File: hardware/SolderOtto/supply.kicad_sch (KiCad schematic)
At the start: 78 parts, among them J201 Conn_02x04_Counter_Clockwise, Q201 T2N7002AK, Q202 BC858B, Q203 BC847A, Q204 BC847A, U201 LM5012, U202 AP3211K, U203 AP3211K, U204 AP3211K, U205 LM27761, U206 MCP9701T-E/TT

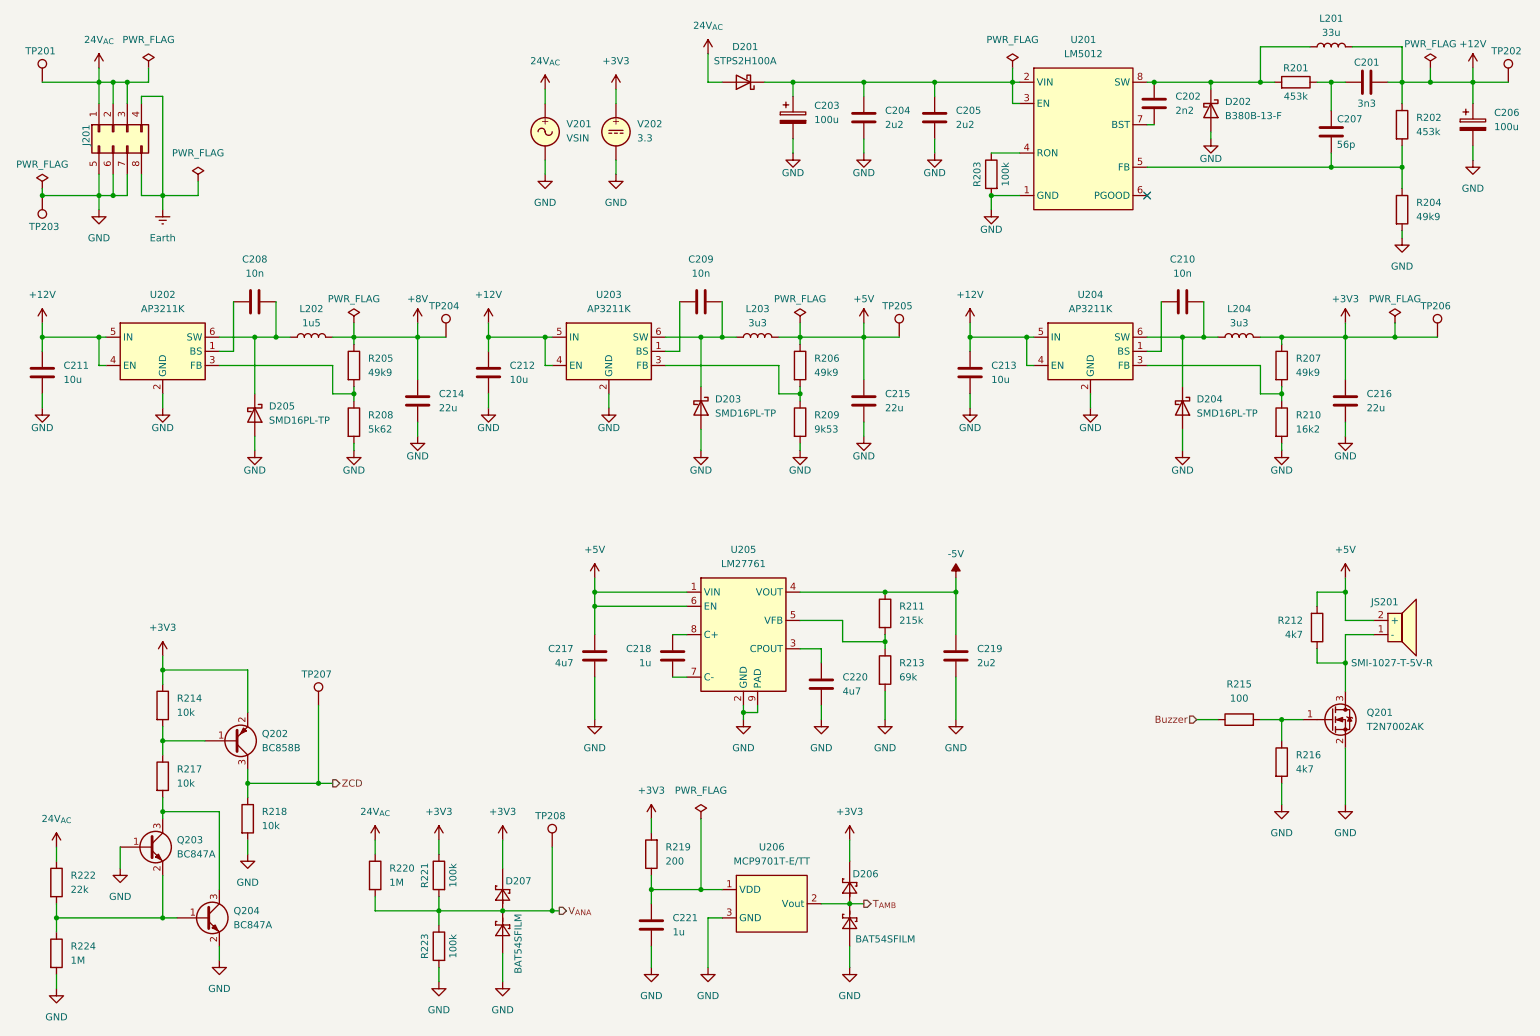
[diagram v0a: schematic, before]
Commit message: start rework supplies
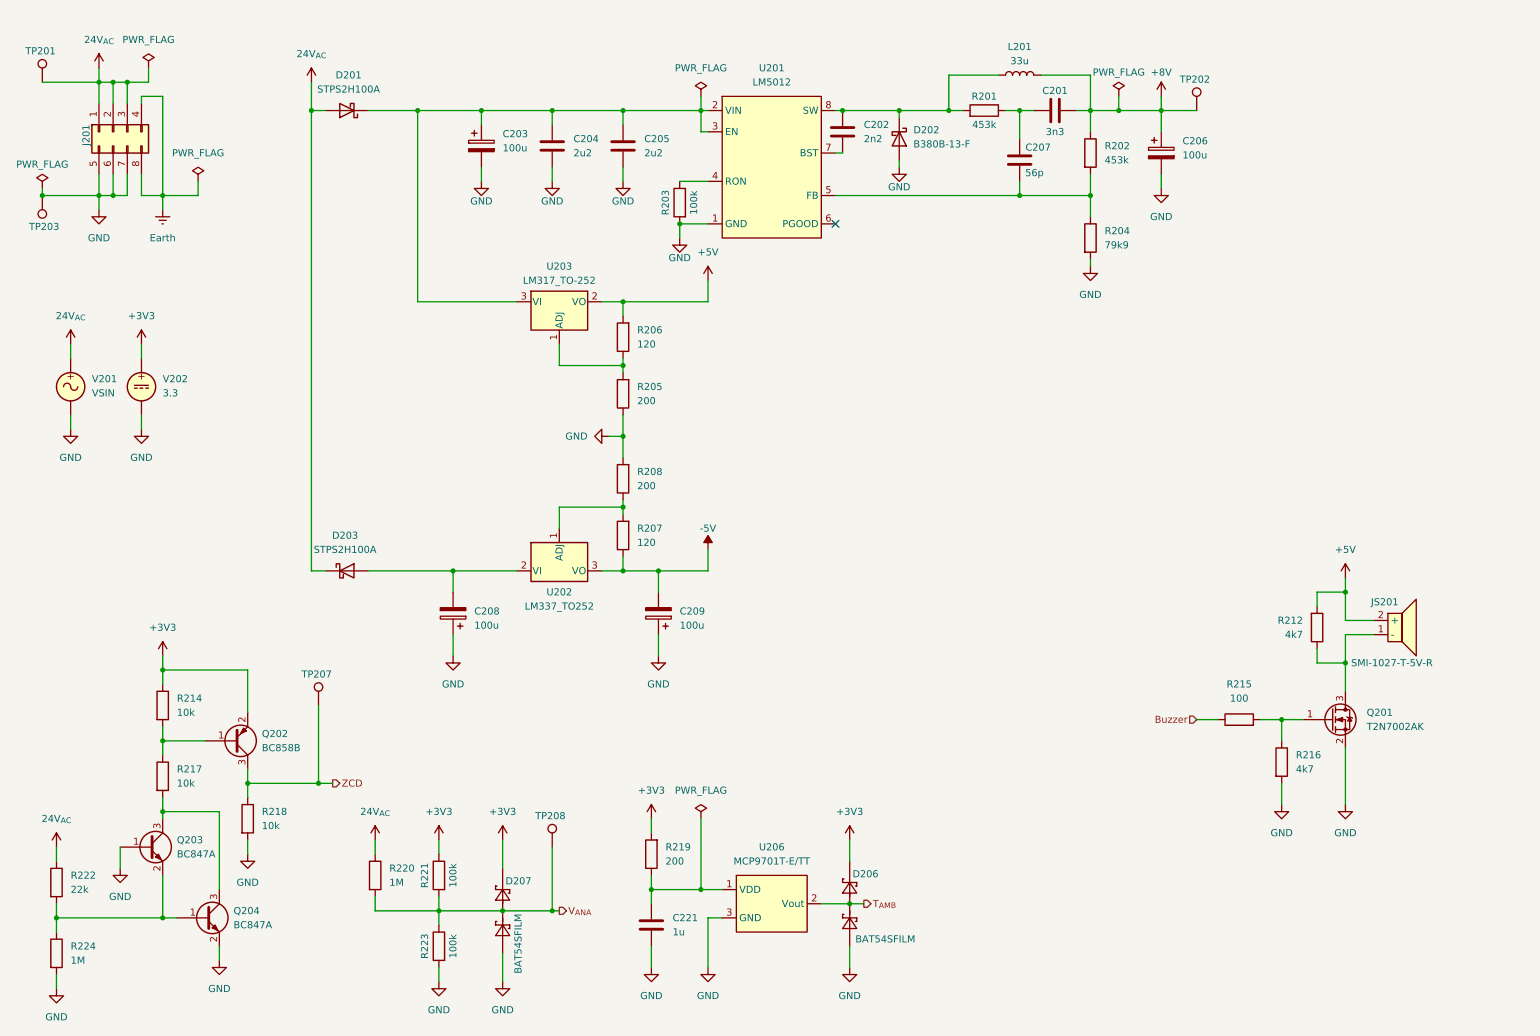
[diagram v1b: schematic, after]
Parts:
- removed C208, C209, C210: 10n, Capacitor_SMD:C_0603_1608Metric, symbol Device:C
- removed C211, C212, C213: 10u, Capacitor_SMD:C_0805_2012Metric, symbol Device:C
- removed C214, C215, C216: 22u, Capacitor_SMD:C_0805_2012Metric, symbol Device:C
- removed C217, C220: 4u7, Capacitor_SMD:C_0603_1608Metric, symbol Device:C
- removed C218: 1u, Capacitor_SMD:C_0603_1608Metric, symbol Device:C
- removed C219: 2u2, Capacitor_SMD:C_0805_2012Metric, symbol Device:C
- removed D204, D205: SMD16PL-TP, Diode_SMD:D_SOD-123F, symbol Device:D_Schottky
- removed L202: 1u5, Inductor_SMD:L_Taiyo-Yuden_NR-40xx, symbol Device:L
- removed L203, L204: 3u3, Inductor_SMD:L_Taiyo-Yuden_NR-40xx, symbol Device:L
- removed R209: 9k53, Resistor_SMD:R_0603_1608Metric, symbol Device:R
- removed R210: 16k2, Resistor_SMD:R_0603_1608Metric, symbol Device:R
- removed R211: 215k, Resistor_SMD:R_0603_1608Metric, symbol Device:R
- removed R213: 69k, Resistor_SMD:R_0603_1608Metric, symbol Device:R
- removed TP204: 8V, TestPoint:TestPoint_Keystone_5015_Micro-Minature, symbol Connector:TestPoint
- removed TP205: 5V, TestPoint:TestPoint_Keystone_5015_Micro-Minature, symbol Connector:TestPoint
- removed TP206: 3V3, TestPoint:TestPoint_Keystone_5015_Micro-Minature, symbol Connector:TestPoint
- removed U202, U203, U204: AP3211K, Package_TO_SOT_SMD:SOT-23-6, symbol Regulator_Switching:AP3211K
- removed U205: LM27761, Package_SON:WSON-8-1EP_2x2mm_P0.5mm_EP0.9x1.6mm, symbol Regulator_SwitchedCapacitor:LM27761
- added C208, C209: 100u, mylib_common:CP_Elec_10x10.5_A768, symbol Device:C_Polarized
- added U202: LM337_TO252, Package_TO_SOT_SMD:TO-252-2, symbol Regulator_Linear:LM337_TO252
- added U203: LM317_TO-252, Package_TO_SOT_SMD:TO-252-2, symbol Regulator_Linear:LM317_TO-252
- D203: value SMD16PL-TP -> STPS2H100A; footprint Diode_SMD:D_SOD-123F -> Diode_SMD:D_SMA; Digikey SMD16PL-TPMSCT-ND -> 497-3758-1-ND
- R204: value 49k9 -> 79k9; Digikey RMCF0603FT49K9CT-ND -> (none)
- R205: value 49k9 -> 200; Digikey RMCF0603FT49K9CT-ND -> (none)
- R206, R207: value 49k9 -> 120; Digikey RMCF0603FT49K9CT-ND -> (none)
- R208: value 5k62 -> 200; Digikey 311-5.62KHRCT-ND -> (none)
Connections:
- net +12V is gone; now on net +8V: C201.2, C206.1, L201.2, R202.1, TP202.1
- net +3V3: no longer R207.1
- net +5V: now also R206.2, U203.2 (VO); no longer R206.1
- net +8V: no longer R205.1
- net -5V: now also R207.1, C209.2, U202.3 (VO)
- net 24V_{AC}: now also D203.1 (K)
- net GND: now also R205.1, C208.1, C209.1; no longer D203.2 (A)
- net at R207.2: now also R208.1, U202.1 (ADJ)
- net at C203.1, C204.1, C205.1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: now also U203.3 (VI)
- net at R205.2: now also R206.1, U203.1 (ADJ); no longer R208.1
- new net: C208.2, D203.2 (A), U202.2 (VI)
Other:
- moved on the sheet: C201, C202, C203, C204, C205, C206, C207, D201, D202, L201, R201, R202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
